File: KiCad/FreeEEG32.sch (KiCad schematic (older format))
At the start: 31 parts, among them P11 CONN_01X03, SW1 NRST, U1 ADP7118AUJZ-3.3_TSOT, U2 ADP7118AUJZ-3.3_TSOT, U3 8.192MHz, U37 STM32F427ZI_4side_short, U39 ADP7118AUJZ-3.3_TSOT, U4 STM32F427ZI_4side, U43 473521001, Y1 32.768kHz, Y2 8MHz

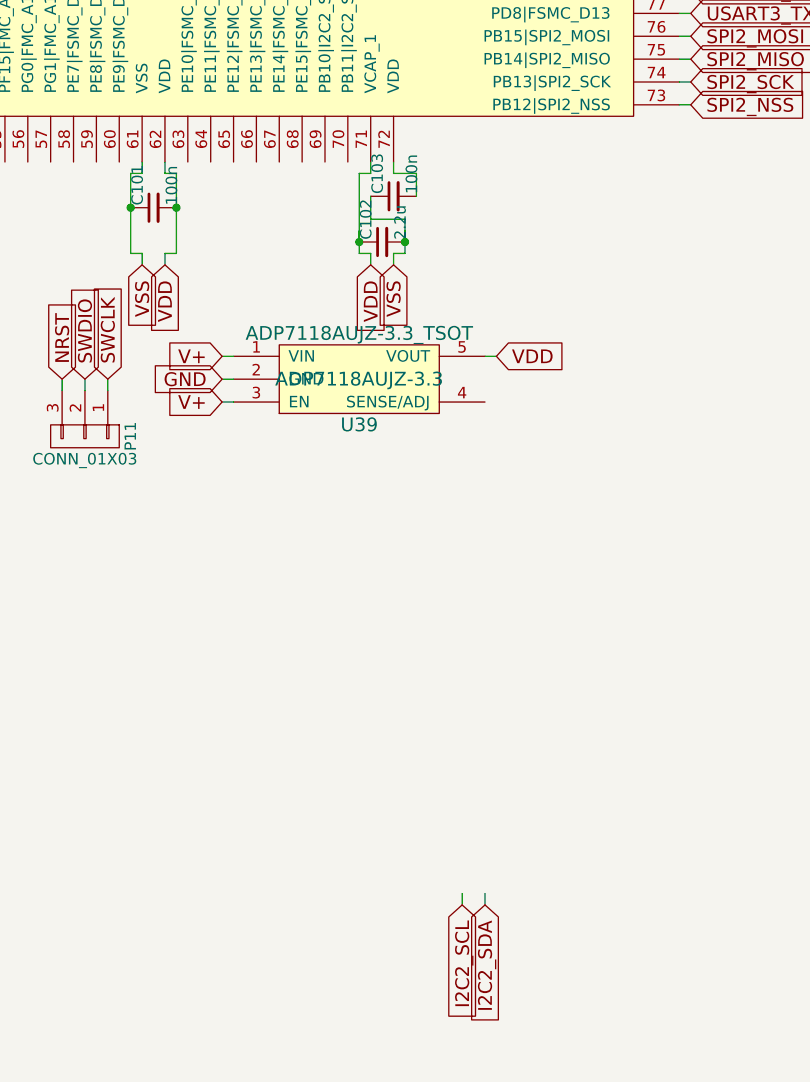
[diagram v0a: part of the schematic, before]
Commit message: kicad
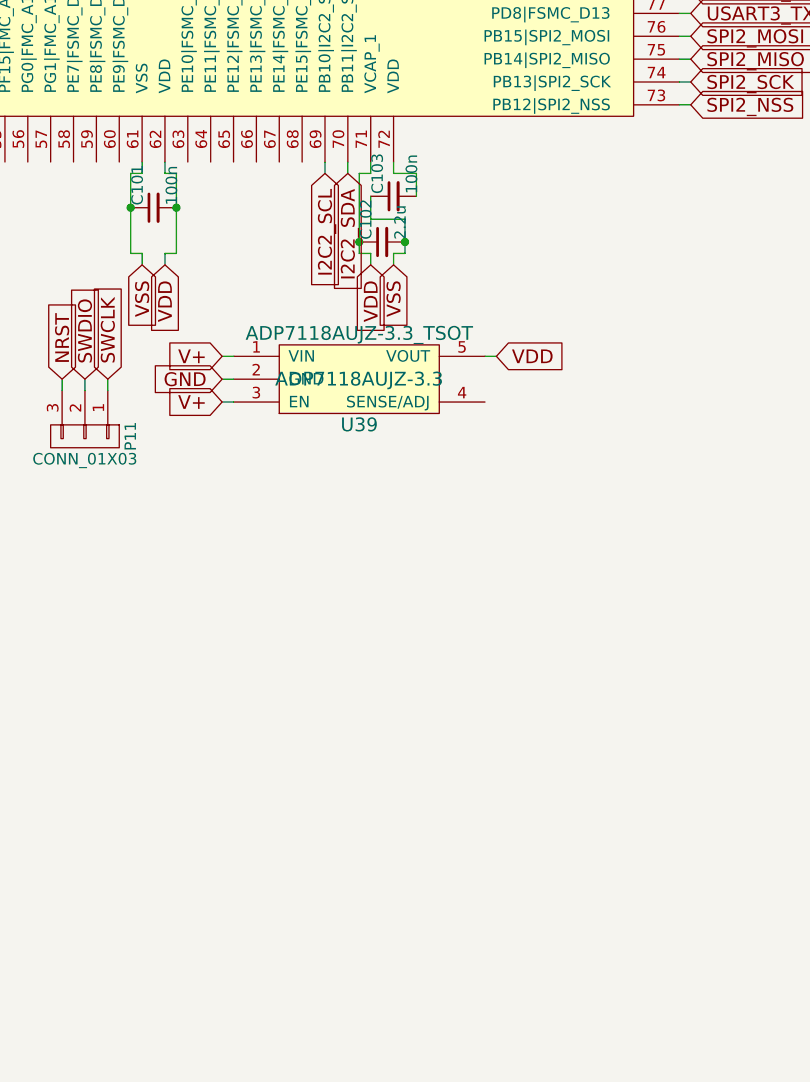
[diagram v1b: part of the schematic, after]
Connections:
- wire segments 302 -> 300
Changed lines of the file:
@@
 	1    0    0    -1
 $EndComp
-Text GLabel 9650 8450 3    60   Input ~ 0
+Text GLabel 9050 5250 3    60   Input ~ 0
 I2C2_SDA
-Text GLabel 9550 8450 3    60   Input ~ 0
+Text GLabel 8950 5250 3    60   Input ~ 0
 I2C2_SCL
 $Comp
@@
 	10900 2850 10950 2850
 Wire Wire Line
-	9300 5500 9300 5600
-Wire Wire Line
-	9100 5500 9100 5600
-Wire Wire Line
-	9100 5550 9100 5250
-Connection ~ 9100 5550
-Connection ~ 9300 5550
+	9100 5250 9100 5600
 Wire Wire Line
 	9100 5250 9150 5250
@@
 	10900 1550 10950 1550
 Wire Wire Line
-	9300 5550 9300 5450
+	9300 5450 9300 5600
 Wire Wire Line
 	9300 5450 9150 5450
@@
 	8500 6250 8550 6250
 Wire Wire Line
-	9550 8450 9550 8400
-Wire Wire Line
-	9650 8450 9650 8400
+	8950 5250 8950 5200
+Wire Wire Line
+	9050 5250 9050 5200
 $Sheet
 S 600  4450 1100 900
@@
 Wire Wire Line
 	10900 3950 10950 3950
+Connection ~ 9300 5550
+Connection ~ 9100 5550
 $EndSCHEMATC

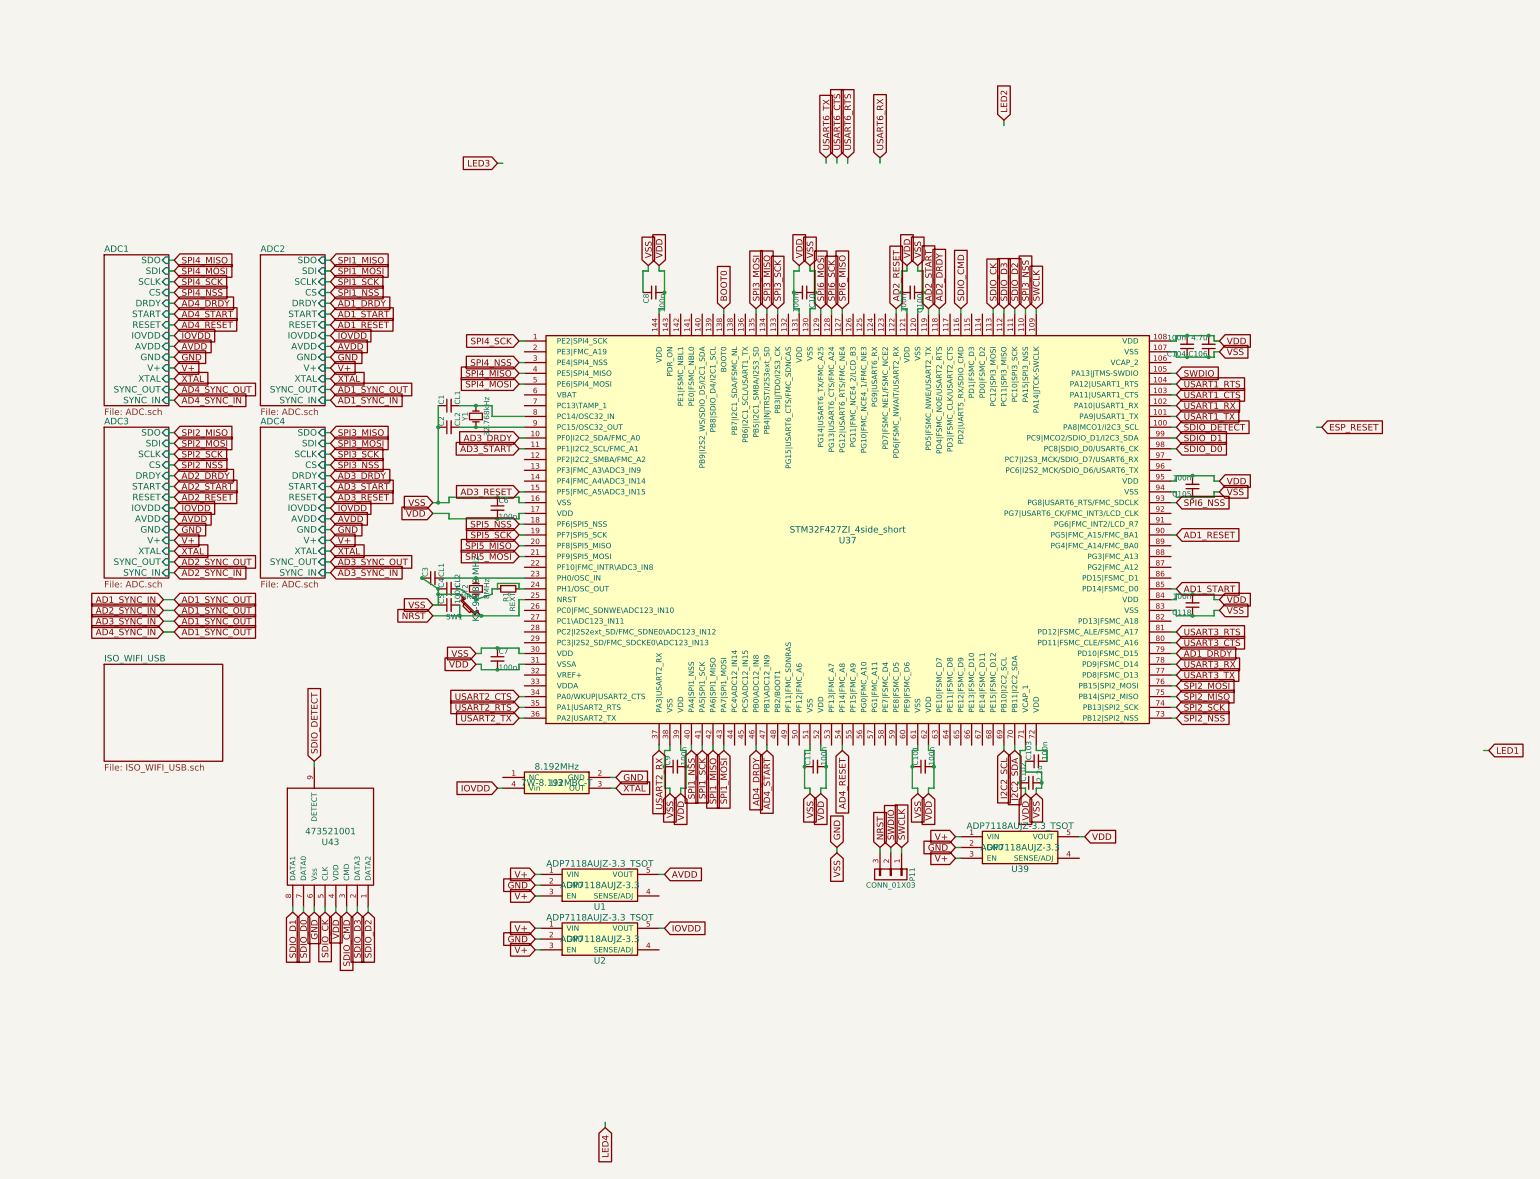
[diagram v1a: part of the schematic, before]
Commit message: kicad
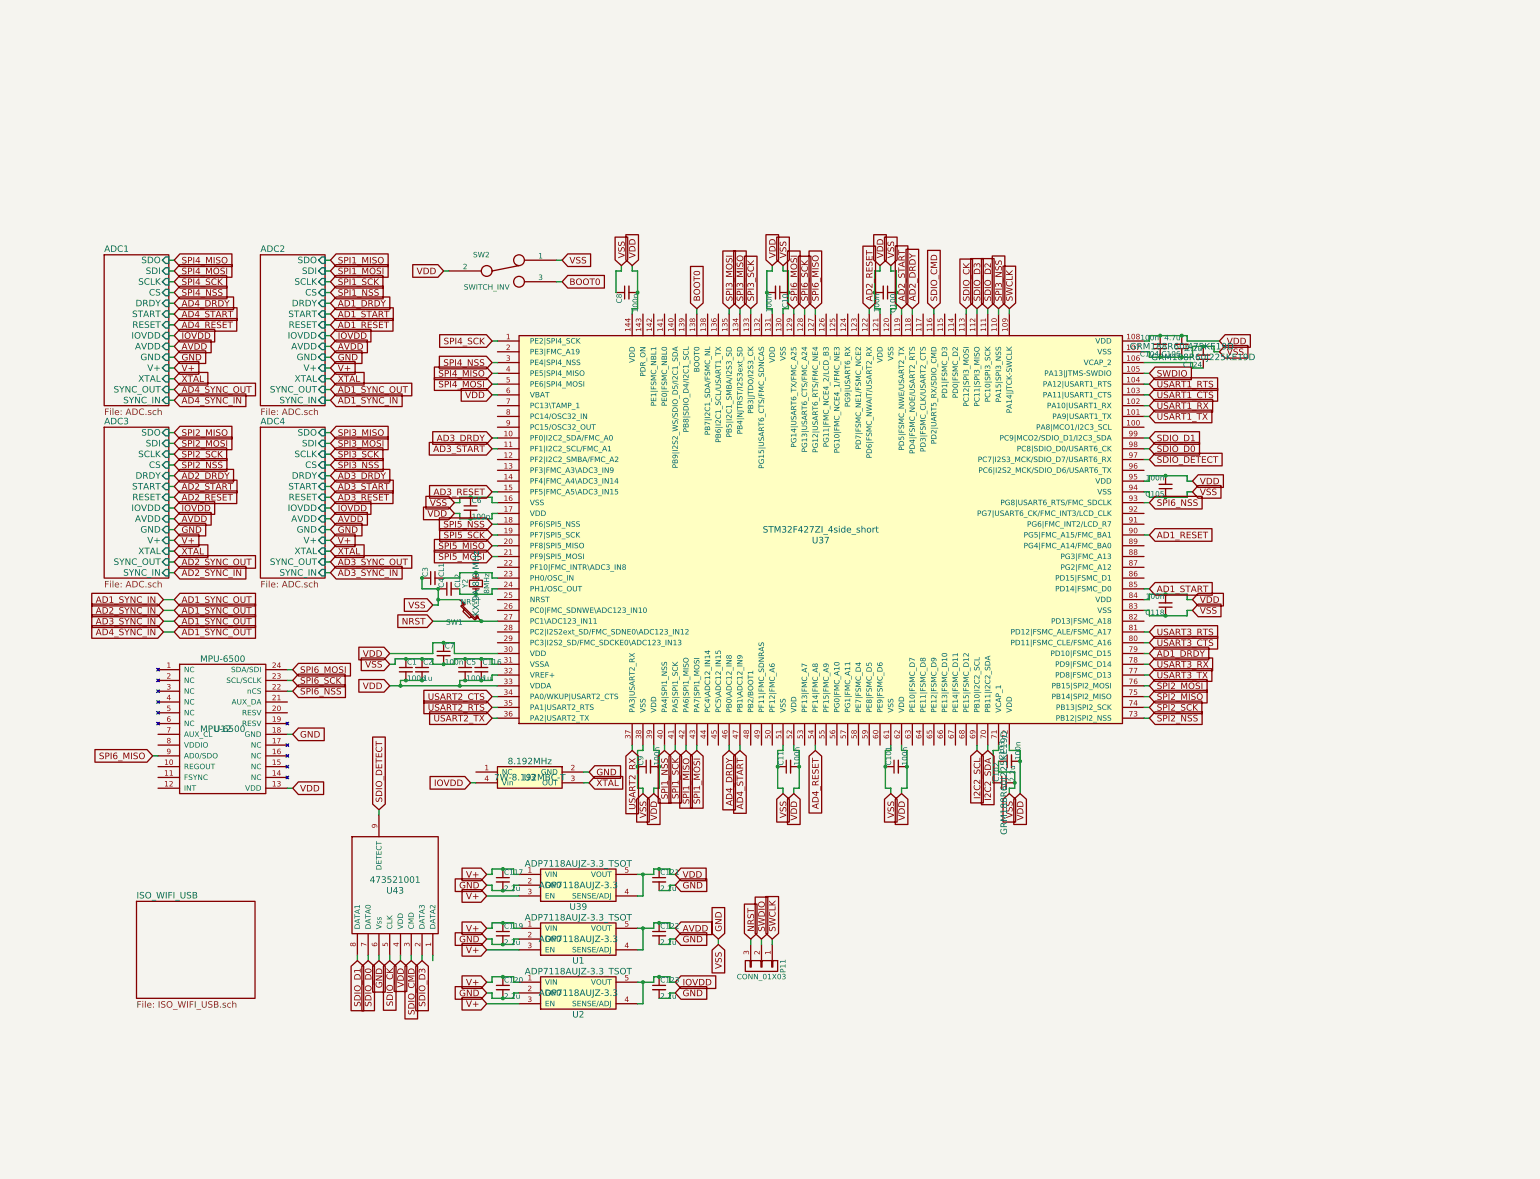
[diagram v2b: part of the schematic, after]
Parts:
- removed R1: REXT, Resistors_SMD:R_0402, symbol R_Small
- removed Y1: 32.768kHz, Crystals:Crystal_SMD_0603_2Pads_obsolete, symbol Crystal_Small
- added C116: 1u, Capacitors_SMD:C_0402, symbol C_Small
- added C117, C119, C120, C121, C122, C123, C124: 2.2u, Capacitors_SMD:C_0603, symbol C_Small
- added SW2: SWITCH_INV, Buttons_Switches_SMD:SW_SPST_B3U-1100P-B, symbol SWITCH_INV
- added U12: MPU-6500, Housings_DFN_QFN:QFN-24-1EP_4x4mm_Pitch0.5mm, symbol MPU-6500
- C1: value CL1 -> 100n
- C102: footprint Capacitors_SMD:C_0402 -> Capacitors_SMD:C_0603; manf# (none) -> GRM188R60J225KE19D
- C106: footprint Capacitors_SMD:C_0402 -> Capacitors_SMD:C_0603; manf# (none) -> GRM188R60J475KE19D
- C2: value CL2 -> 1u
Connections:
- net AVDD: now also U1.4 (SENSE/ADJ), C122.1
- net BOOT0: now also SW2.3
- net GND: now also C7.2, U37.31 (VSSA), C116.1, C117.2, C119.2, C120.2, C121.2, C122.2, C123.2, C124.2, SW2.1, U12.18 (GND); no longer C7.1, U37.30 (VDD)
- net IOVDD: now also U2.4 (SENSE/ADJ), C123.1
- net NRST: now also U37.27 (PC1\ADC123_IN11); no longer C5.2, U37.25 (NRST)
- net SDIO_D2: no longer U43.1 (DATA2)
- net SDIO_DETECT: now also U37.97 (PC7|I2S3_MCK/SDIO_D7/USART6_RX); no longer U37.100 (PA8|MCO1/I2C3_SCL)
- net SPI6_MISO: now also U12.9 (AD0/SDO)
- net SPI6_MOSI: now also U12.24 (SDA/SDI)
- net SPI6_NSS: now also U12.22 (nCS)
- net SPI6_SCK: now also U12.23 (SCL/SCLK)
- net V+: now also C117.1, C119.1, C120.1
- net VDD: now also C1.2, C103.2, C2.2, C5.2, C7.1, U37.30 (VDD), U37.32 (VREF+), U37.33 (VDDA), U37.6 (VBAT), U37.72 (VDD), U39.4 (SENSE/ADJ), C116.2, C121.1, SW2.2, U12.13 (VDD); no longer C102.1, C7.2, U37.31 (VSSA), U37.71 (VCAP_1)
- net at U37.9 (PC15/OSC32_OUT): no longer C2.2
- net at U37.8 (PC14/OSC32_IN): no longer C1.2
- net at U37.106 (VCAP_2): now also C124.1
- new net: C102.1, U37.71 (VCAP_1)
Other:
- moved on the sheet: C10, C100, C101, C102, C103, C104, C105, C106, C11, C118, C6, C7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

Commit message: kicad
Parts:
- removed U4: STM32F427ZI_4side, symbol STM32F427ZI_4side
- C1, C10, C100, C101, C103, C104, C105, C11, C118, C5, C6, C7, C8, C9: manf# (none) -> MC0402B104K160CT
- C116, C2: manf# (none) -> GRM155R60J105KE19D
- C117, C119, C120, C121, C122, C123: manf# (none) -> GRM188R60J225KE19D
- P11: manf# (none) -> PBS-3
- U3: manf# 7W-8.192MBC-T -> 7W-8.192MBA-T
- U43: manf# (none) -> 473521001
